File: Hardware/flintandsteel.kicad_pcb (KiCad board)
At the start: 4 copper layers, 145 parts, among them J1 RBUS, J2 USB_C_Receptacle_USB2.0, J3 Conn_01x02_Male, J4 Conn_01x02_Male, J5 Conn_01x02_Male, J6 Conn_01x02_Male, Q1 NCV8403, Q2 NCV8403, Q3 NCV8403, Q4 NCV8403, U1 ESP32-S3, U2 SN65HVD230, U3 LM66200DRLR, U4 MAX77827AEFD+T, U5 SC4215, U6 LTV-247, U7 SiC431, Y1 40MHz±10ppm

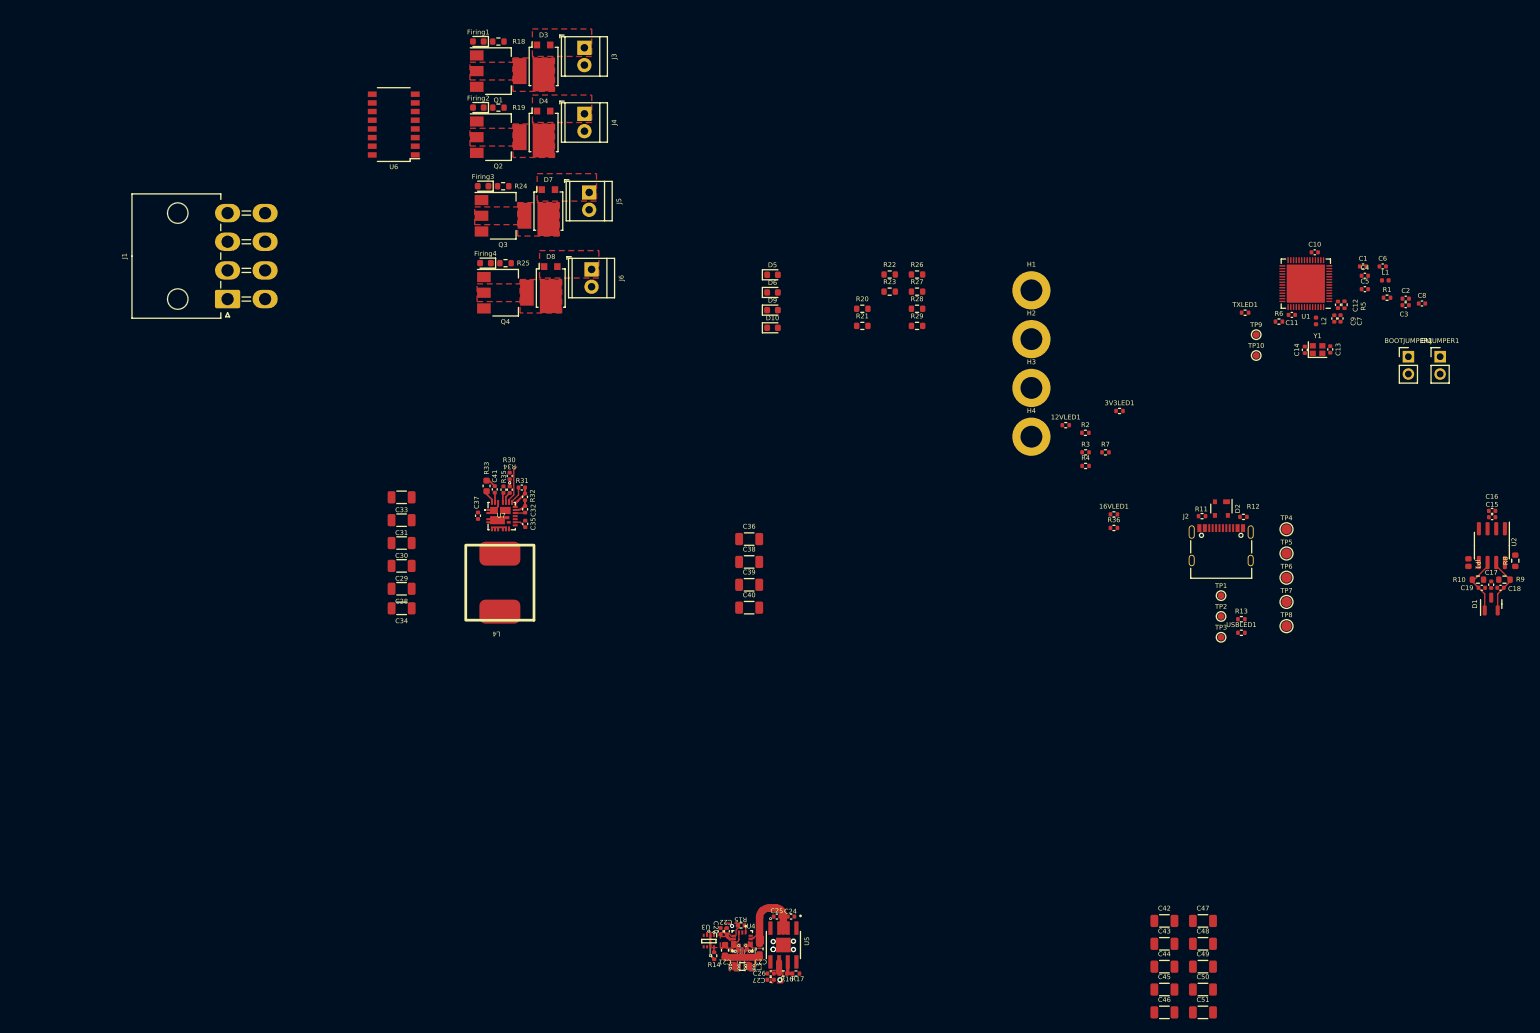
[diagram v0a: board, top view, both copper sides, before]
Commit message: I don't remember what I did but I have to move these files to my desktop
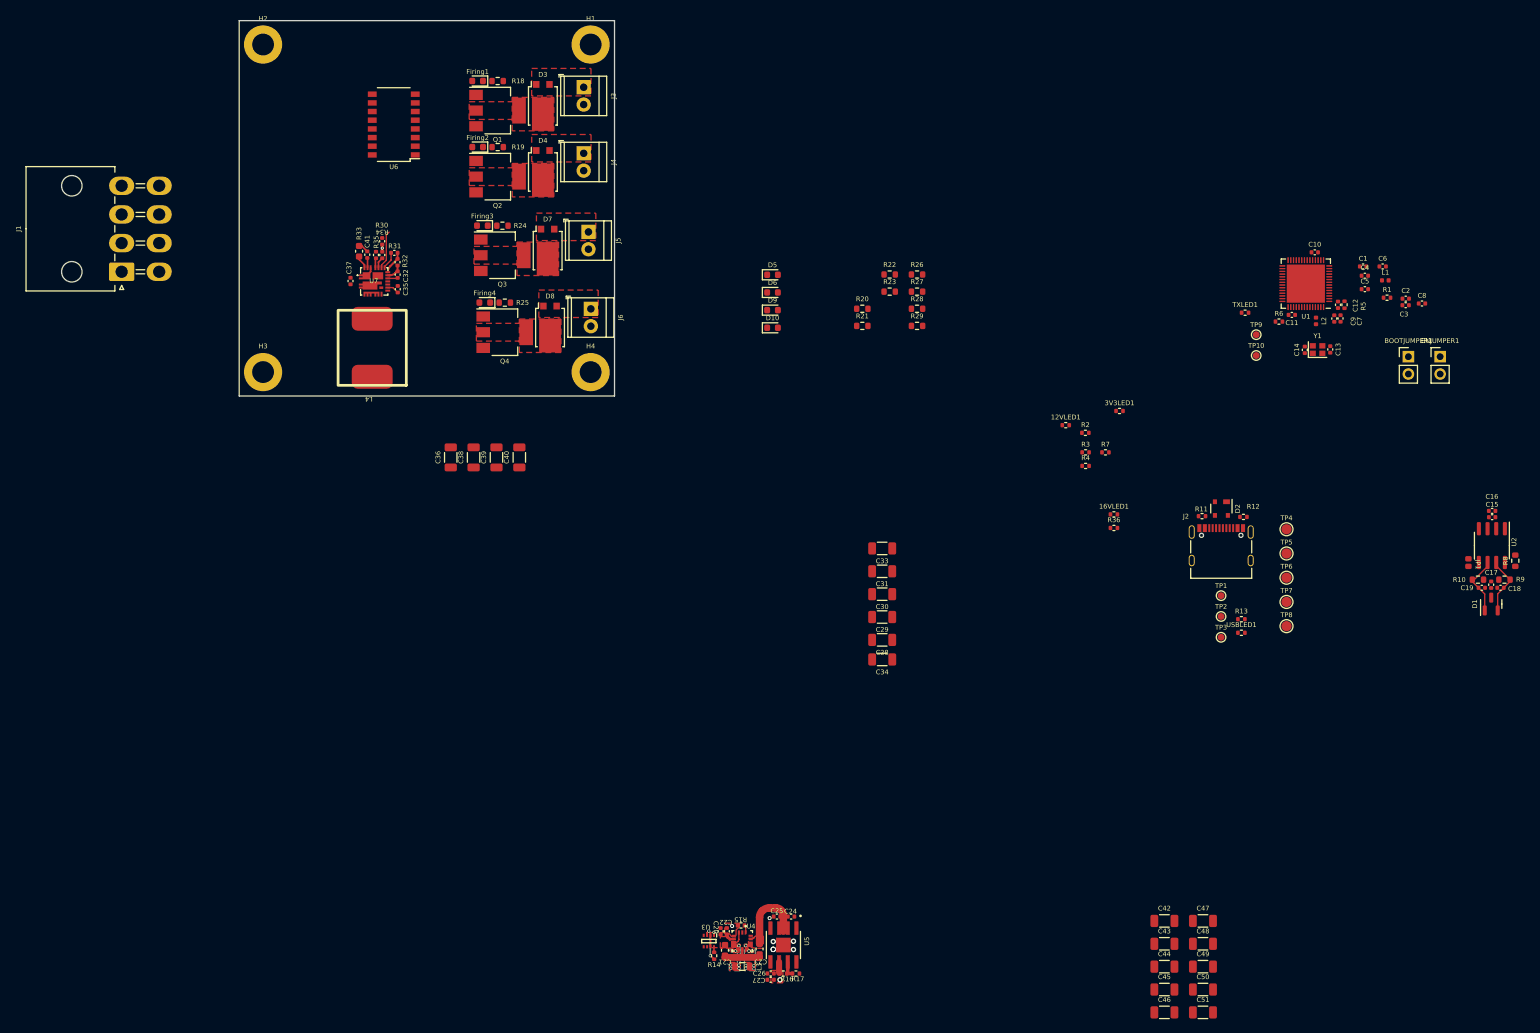
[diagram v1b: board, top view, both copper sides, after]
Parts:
- moved H2 120.6 mm to (60.5, 22.5)
- moved H3 112.6 mm to (60.5, 70.5)
- moved H1 74.0 mm to (108.5, 22.5)
- moved C28 70.8 mm to (151.2, 109.7)
- moved C29 70.8 mm to (151.2, 106.4)
- moved C30 70.8 mm to (151.2, 103.0)
- moved C31 70.8 mm to (151.2, 99.7)
- moved C33 70.8 mm to (151.2, 96.3)
- moved C34 70.8 mm to (151.2, 112.6)
- moved H4 65.3 mm to (108.5, 70.5)
- moved C36 45.3 mm to (88.0, 83.0), turned to 90 degrees
- moved C38 43.2 mm to (91.3, 83.0), turned to 90 degrees
- moved C39 41.5 mm to (94.7, 83.0), turned to 90 degrees
- moved C40 40.2 mm to (98.0, 83.0), turned to 90 degrees
- moved L4 39.2 mm to (81.5, 72.4)
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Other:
- board outline added: 55 x 55 mm
